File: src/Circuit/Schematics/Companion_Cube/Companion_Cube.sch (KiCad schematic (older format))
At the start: 15 parts, among them CON1 AVR-ISP-6, IC1 ATTINY85-S, P1 CONN_11, U1 MINI-B_USB

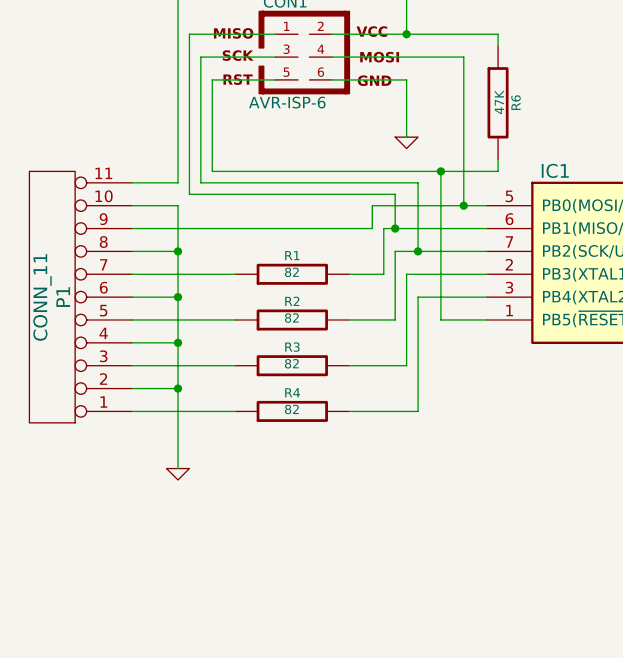
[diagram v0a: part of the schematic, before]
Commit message: Redesigning circuit board for new model
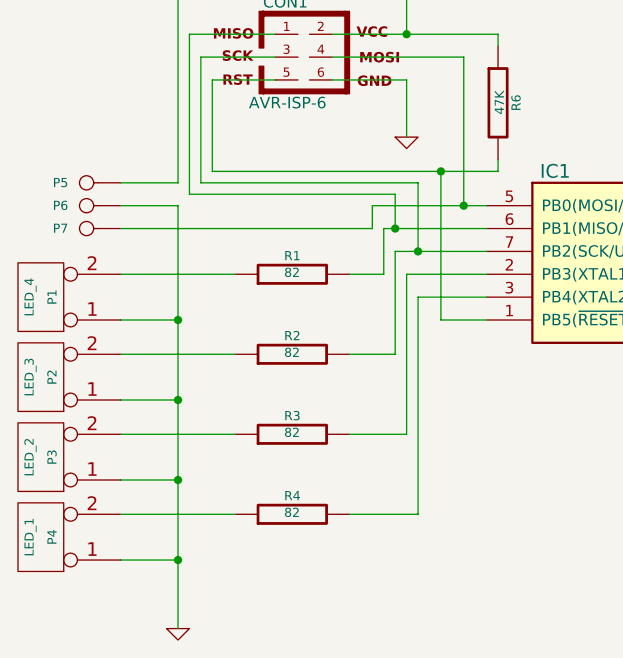
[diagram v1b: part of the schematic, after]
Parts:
- removed P1: CONN_11, ~, symbol CONN_11
- added P1: LED_4, ~, symbol CONN_2
- added P2: LED_3, ~, symbol CONN_2
- added P3: LED_2, ~, symbol CONN_2
- added P4: LED_1, ~, symbol CONN_2
- added P5, P6, P7: CONN_1, ~, symbol CONN_1
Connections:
- net GND: now also P1.1 (P1), P2.1 (P1), P3.1 (P1), P4.1 (P1), P6.1
- net VCC: now also P5.1
- net at CON1.4, IC1.5 (PB0(MOSI/DI/SDA/AIN0/OC0A/OC1A/AREF/PCINT0)): now also P7.1
- net at R4.1: now also P4.2 (PM)
- net at R3.1: now also P3.2 (PM)
- net at R2.1: now also P2.2 (PM)
- net at R1.1: now also P1.2 (PM)
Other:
- moved on the sheet: R2, R3, R4
